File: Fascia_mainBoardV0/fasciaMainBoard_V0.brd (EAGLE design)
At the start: 33.6 x 40.6 mm, 114 parts, among them J1 MOLEX_52435-2271MOLEX_52435-2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, J3 -, J8 TC2030-MCP, Q1 BSS138PS,115, U1 ATSAMD21G-A, U10 ADUM5028, U17 MPU-6050, U18 LP5912Q3.3DRVRQ1, U3 NINA-W102, U4 ATECC508A-MAHDA-T, U5 MCP73831T-4ADI_OT, U6 LM2664M6_NOPB, U7 TPS72325QDBVRQ1, U8 TLV70025DDCR, U9 LP5912Q3.3DRVRQ1, Y1 32.768Khz

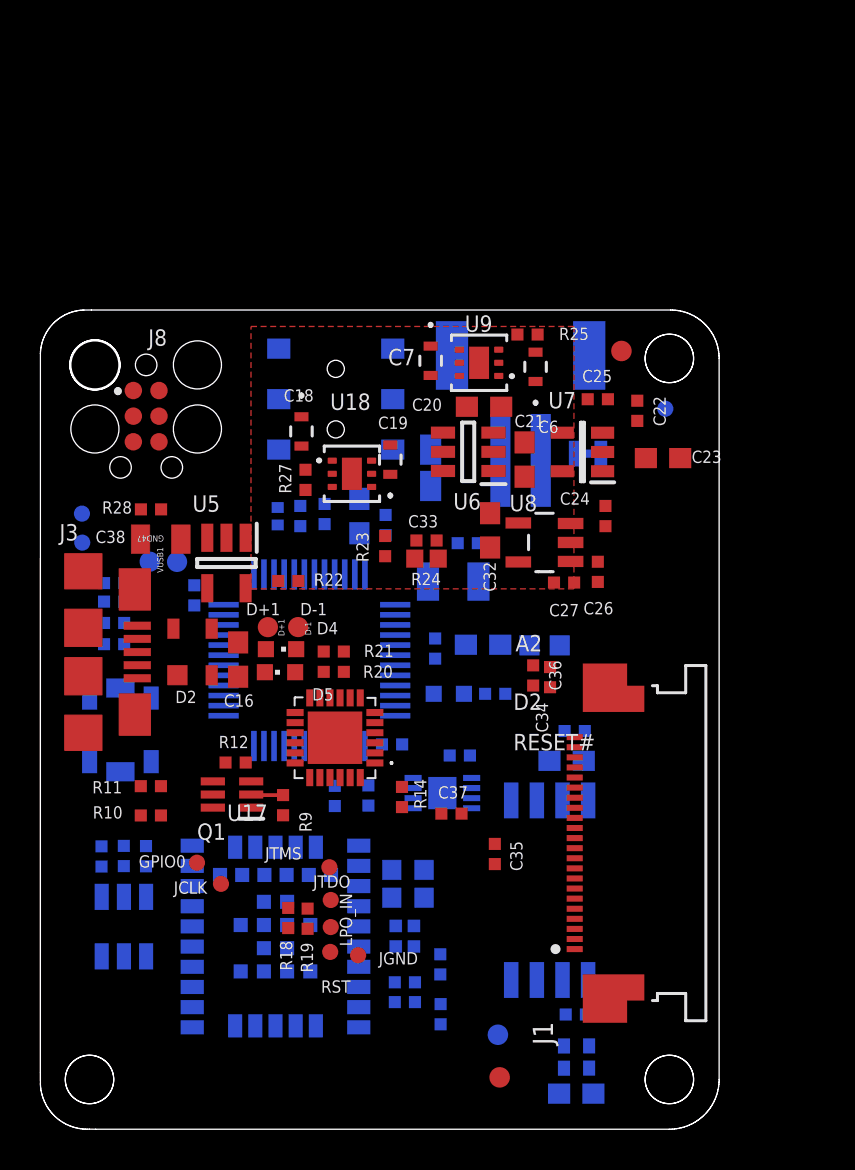
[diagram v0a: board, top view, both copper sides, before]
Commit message: minor updates
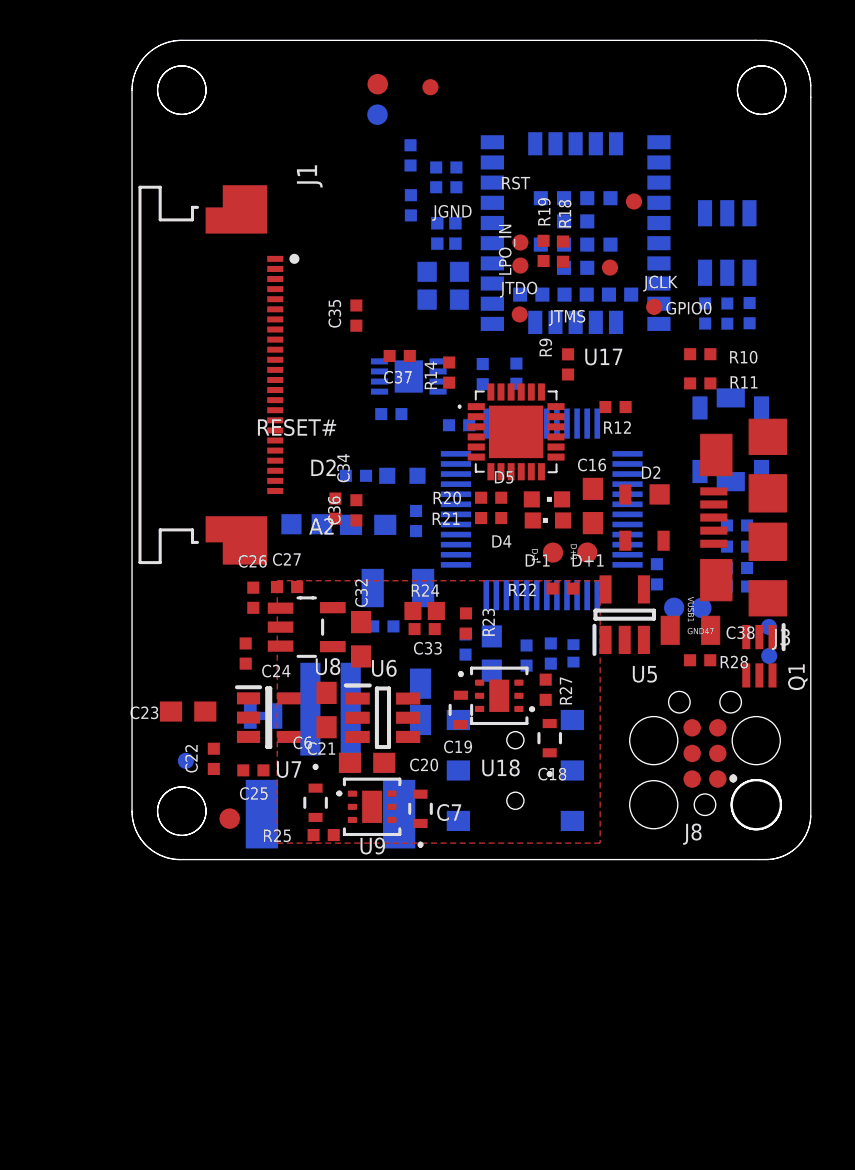
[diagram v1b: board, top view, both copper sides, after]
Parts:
- removed C41, C64: 10uF, SparkFun-Capacitors:0603
- removed C49: 0.1uF, novaXR:0402-TIGHT
- removed C51: 0.22uF, novaXR:0402-TIGHT
- removed L1, L2: BLM15HD182SN1D, SamacSys_Parts:INDC1005X55N
- removed U10: ADUM5028, novaXR:SOIC_IC
- J1: value MOLEX_52435-2271MOLEX_52435-2271_0_0 -> MOLEX_52437-2471MOLEX_52437-2471_0_0; device Molex - 52435-2271:MOLEX_52435-2271_0 -> Molex - 52437-2471:MOLEX_52437-2471_0
- moved FD1 49.6 mm to (35.8, 52.5), turned to 180 degrees
- moved FD3 46.0 mm to (35.8, 51.0), turned to 180 degrees
- moved D3 45.2 mm to (53.1, 44.6), turned to 90 degrees
- moved JGND 43.2 mm to (38.4, 52.4), turned to 270 degrees
- moved R13 42.6 mm to (37.4, 49.0), turned to 90 degrees
- moved R17 41.9 mm to (54.2, 41.2), turned to 270 degrees
- moved C13 41.4 mm to (39.2, 48.4), turned to 180 degrees
- moved U3 40.9 mm to (45.3, 46.8), turned to 90 degrees
- moved R16 40.2 mm to (53.1, 41.1), turned to 270 degrees
- moved RST 40.1 mm to (48.5, 46.7), turned to 180 degrees
- moved C12 39.4 mm to (39.2, 47.4), turned to 0 degrees
- moved R15 38.6 mm to (52.0, 41.1), turned to 270 degrees
- moved R4 37.6 mm to (37.4, 46.5), turned to 270 degrees
- moved JCLK 36.1 mm to (47.3, 43.4), turned to 270 degrees
- moved C28 35.9 mm to (39.2, 45.6), turned to 180 degrees
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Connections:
- new net ADS_CLK: J1.24
- new net BIAS_INV: J1.1
- new net N$14: J1.11
- new net N$22: J1.3
- new net N$24: J1.6
- new net N$26: J1.9
- new net PA07_DRDY2: J1.23
- net ADS_RESET: no longer J1.5
- net ADS_RESET2: now also J1.20
- net AGND: now also J1.8; no longer J1.14, J1.15, J1.16
- net AVDD: now also J1.4; no longer J1.20, J1.21, J1.22
- net AVSS: now also J1.5; no longer J1.17, J1.18, J1.19
- net DVDD: now also J1.10; no longer C41.2, C49.2, J1.11, J1.12, J1.13, U10.3
- net DVDD_ISO: no longer C64.2, L1.2
- net GND: now also J1.13, J1.14, J1.15; no longer C41.1, C49.1, J1.10, J1.8, J1.9, U10.1, U10.2, U10.4
- net GND_ISO: no longer C51.1, C64.1, L2.1, L2.2, U10.5, U10.7, U10.8
- net N$5: now also J1.7; no longer C51.2, L1.1, U10.6
- net PA02_EDA_SIG: now also J1.2; no longer J1.7
- net PA16_S1_MOSI: now also J1.21; no longer J1.6
- net PA17_S1_SCK: now also J1.19; no longer J1.3
- net PA19_S1_MISO: now also J1.18; no longer J1.2
- net PA20_CS2: now also J1.22
- net PA21_CS1: no longer J1.4
- net PB10_DRDY: no longer J1.1
- net S0_I2C_SCL: now also J1.16
- net S0_I2C_SDA: now also J1.17
- net VCC: now also J1.12
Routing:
- net PB08_RST: track 1.59 -> 0.00 mm
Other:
- outline, holes or cut-outs redrawn
